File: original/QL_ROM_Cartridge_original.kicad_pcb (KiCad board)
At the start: 2 copper layers, 38.6 x 84.8 mm, 6 parts, among them IC1 27C128, IC2 27C128, IC3 74LS00, J1 QL_cartridge_ROM

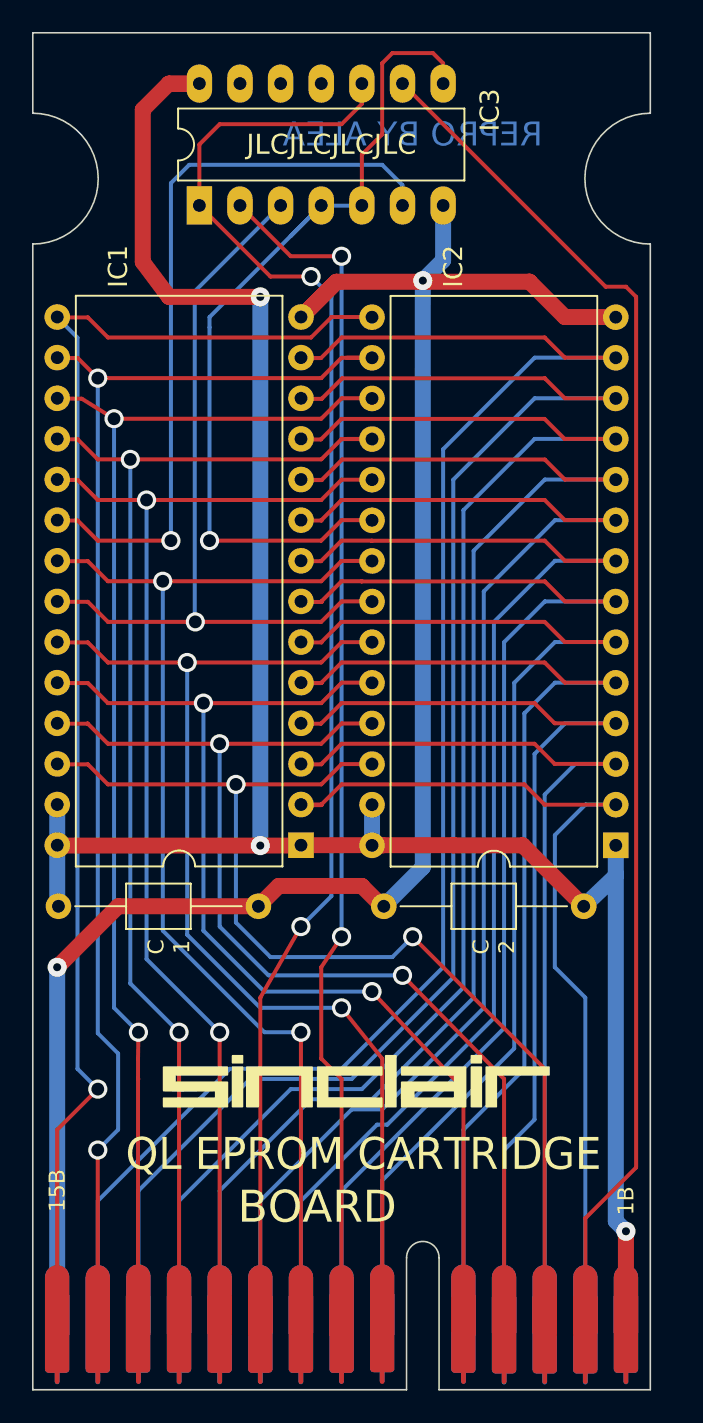
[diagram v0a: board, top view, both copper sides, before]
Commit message: update
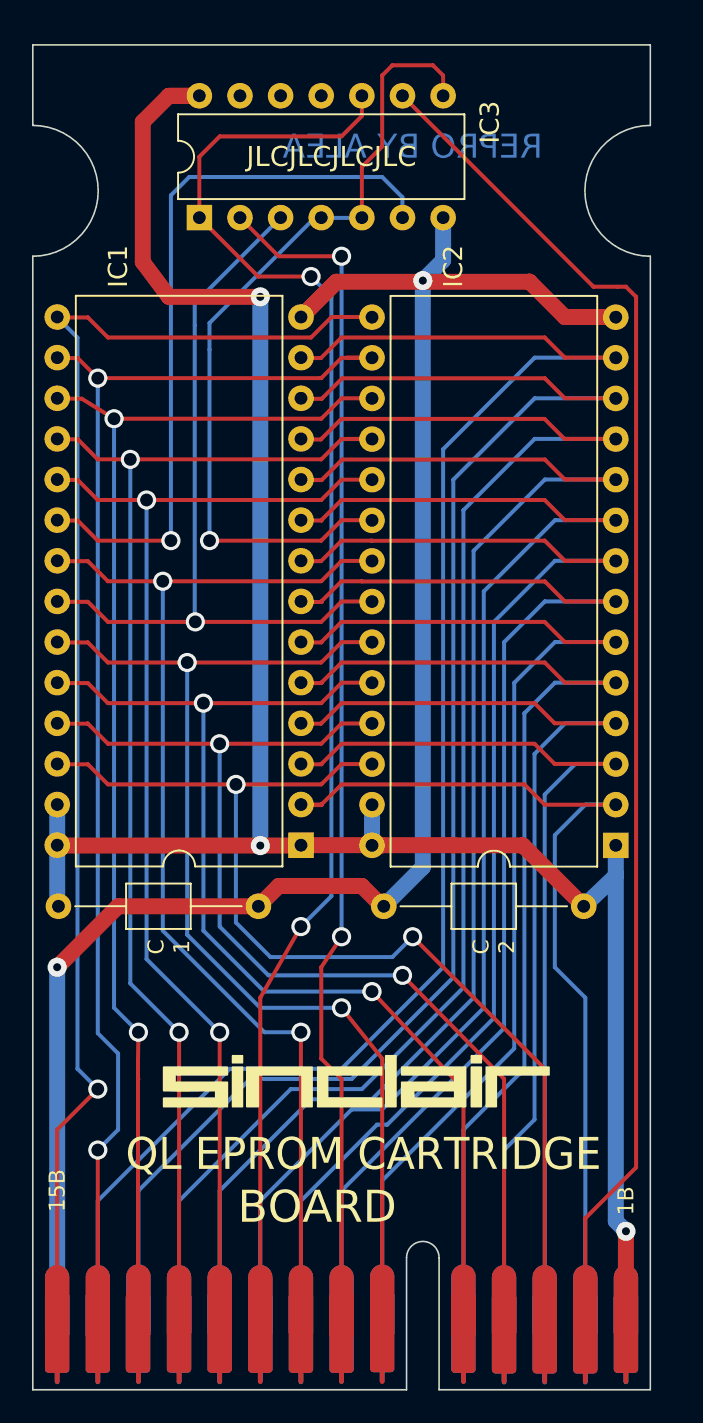
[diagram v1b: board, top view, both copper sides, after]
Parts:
- IC3: footprint Package_DIP:DIP-14_W7.62mm_LongPads -> Package_DIP:DIP-14_W7.62mm
- moved IC3 0.76 mm to (72.4, 71.2)
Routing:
- net /U2_CE: track 53.7 -> 50.5 mm
- net VCC: track 131.0 -> 130.2 mm
- net GND: track 114.2 -> 113.4 mm
- net /U_ROMOE: track 48.4 -> 47.6 mm
- net /U1_CE: track 46.7 -> 46.0 mm
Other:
- board size 38.6 x 84.8 mm -> 38.6 x 84.1 mm

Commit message: Updated Original PCB
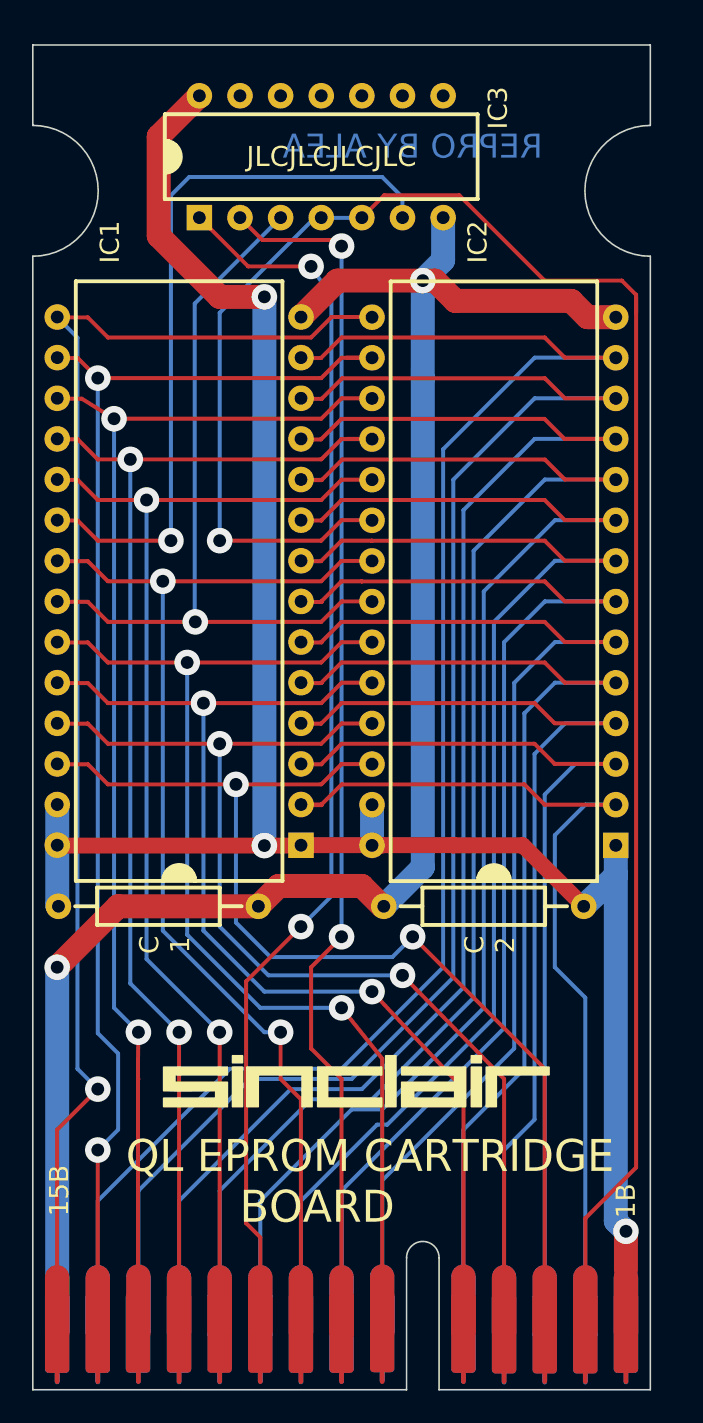
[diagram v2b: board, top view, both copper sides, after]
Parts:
- C1: footprint Capacitor_THT:C_Axial_L3.8mm_D2.6mm_P12.50mm_Horizontal -> 8bits:C_Axial_L3.8mm_D2.6mm_P12.50mm_Horizontal_Sinclair_Cartridge
- IC1: footprint Package_DIP:DIP-28_W15.24mm -> 8bits:DIP-28_W15.24mm_sinclair_cartridge
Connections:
- net /U1_CE renamed /NOT_A14
- IC2 pad 20: /U2_CE -> /A14
- IC3 pad 10: /A15 -> unconnected-(IC3-Pad10)
- IC3 pad 4: /U2_CE -> /A14
- IC3 pad 5: /U2_CE -> /A14
- IC3 pad 8: /U2_CE -> unconnected-(IC3-Pad8)
- IC3 pad 9: /A14 -> unconnected-(IC3-Pad9)
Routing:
- net /U2_CE: track 50.5 -> 0.00 mm, vias 1 -> 0
- net /A14: track 82.0 -> 117.8 mm, vias 0 -> 1
- net /A15: track 89.4 -> 76.1 mm
- net VCC: track 130.2 -> 124.8 mm
- net GND: track 113.4 -> 110.3 mm
- net /ROMOE: track 71.6 -> 72.7 mm
- net /A10: track 70.3 -> 71.2 mm
